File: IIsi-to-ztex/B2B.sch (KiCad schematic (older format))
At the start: 8 parts, among them J1 Conn_02x07_Odd_Even

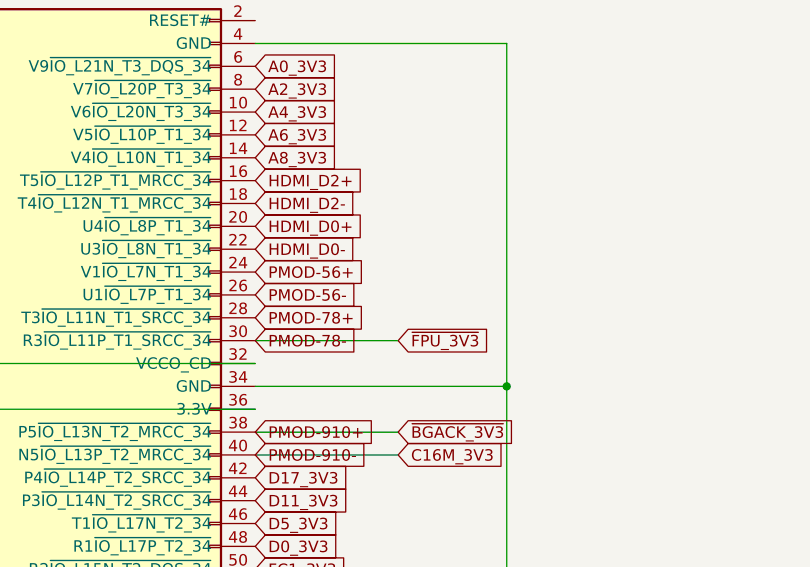
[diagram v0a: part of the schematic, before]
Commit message: cleanup DRC
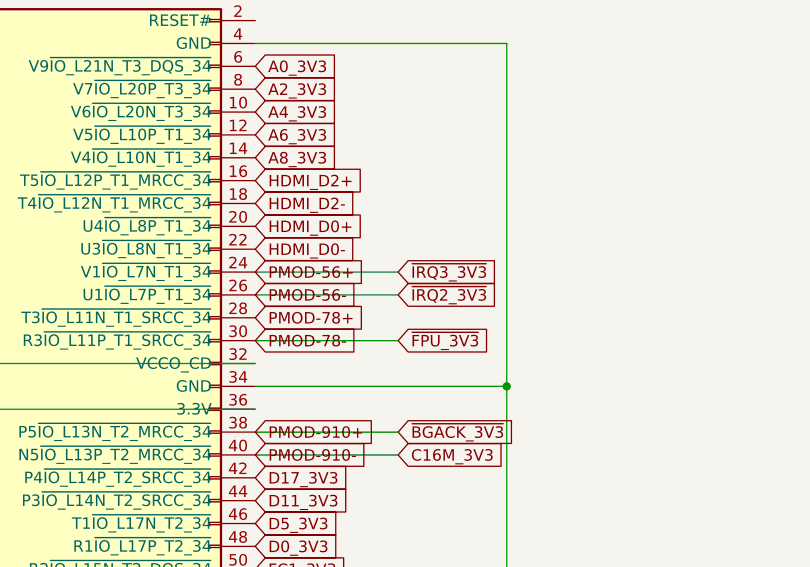
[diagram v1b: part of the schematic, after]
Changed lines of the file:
@@
 Wire Wire Line
 	9900 2550 10525 2550
+Text GLabel 10525 2250 2    50   Input ~ 0
+~IRQ3_3V3
+Text GLabel 10525 2350 2    50   Input ~ 0
+~IRQ2_3V3
+Wire Wire Line
+	9900 2350 10525 2350
+Wire Wire Line
+	10525 2250 9900 2250
 $EndSCHEMATC
